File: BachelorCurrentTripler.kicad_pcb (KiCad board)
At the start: 2 copper layers, 132.3 x 99.3 mm, 54 parts, among them Q13 C2M0025120D, Q14 C2M0025120D, Q15 C2M0025120D, Q16 C2M0025120D, Q7 C2M0025120D, Q8 C2M0025120D, U1 STDriveG600, U2 STDriveG600, U3 STDriveG600

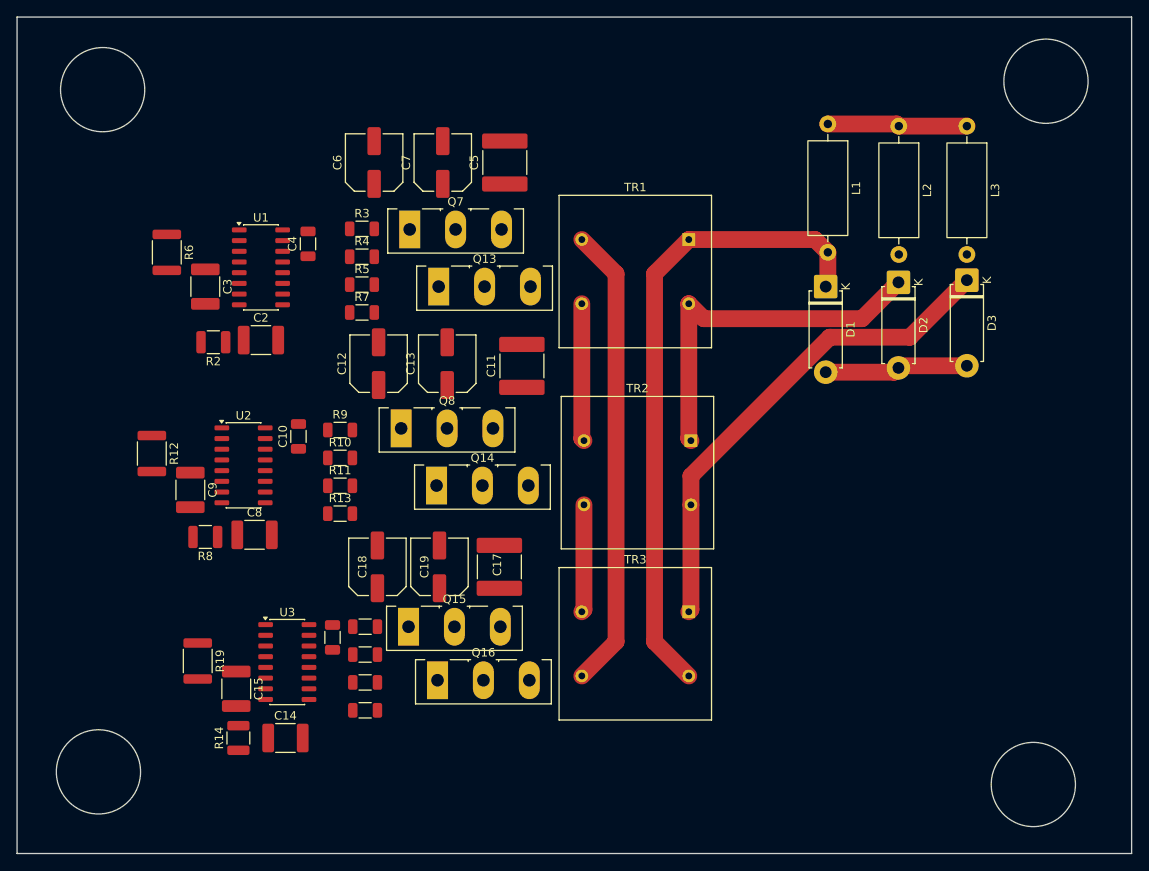
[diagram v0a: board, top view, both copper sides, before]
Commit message: intial pcb layout
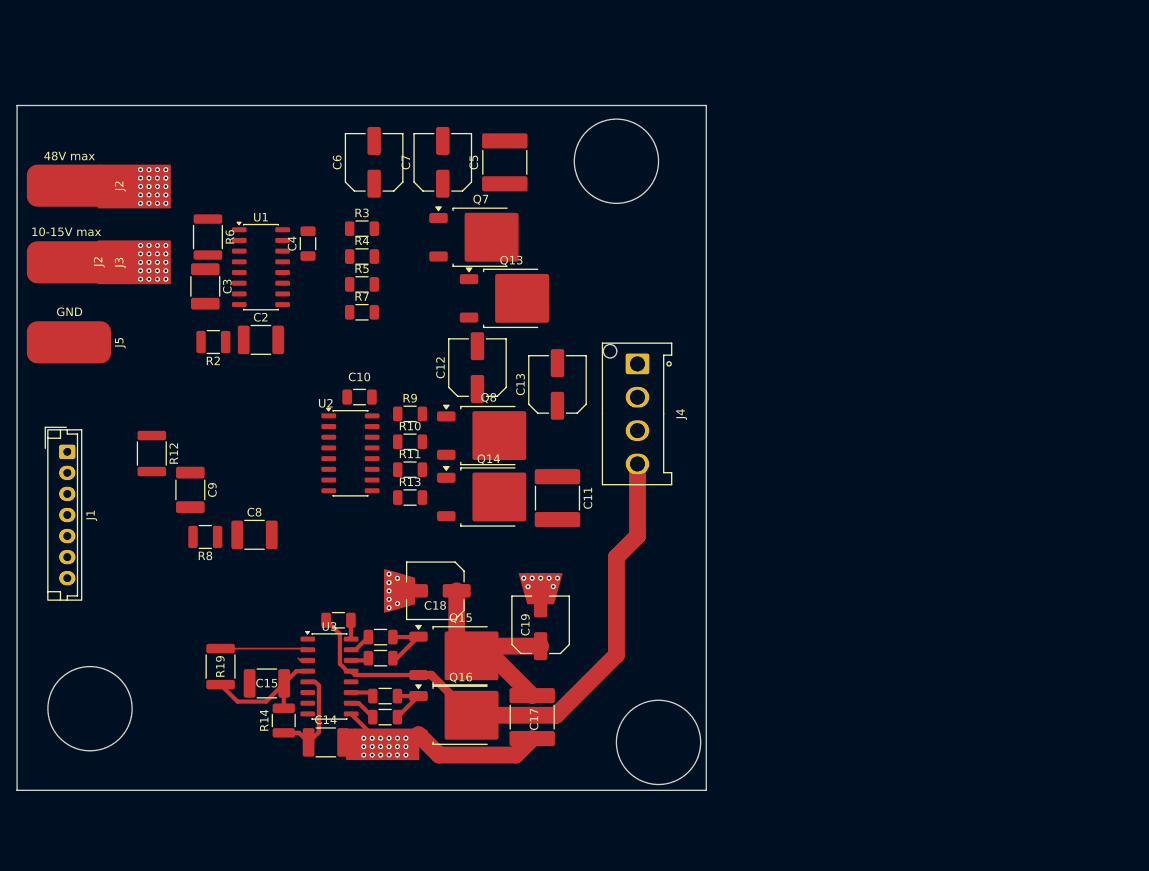
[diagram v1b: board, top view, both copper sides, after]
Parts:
- removed D1, D2, D3: D, Diode_THT:D_5W_P10.16mm_Horizontal
- removed L1, L2, L3: L, Inductor_THT:L_Axial_L11.0mm_D4.5mm_P15.24mm_Horizontal_Fastron_MECC
- removed TR1, TR2, TR3: 48:2, Transformer_THT:Transformer_NF_ETAL_1-1_P1200
- added J1: Conn_01x07_Pin, Connector_JST:JST_EH_B7B-EH-A_1x07_P2.50mm_Vertical, F.Cu at (90.8, 107.5)
- added J2: Conn_01x01_Pin, Connector_Wire:SolderWirePad_1x01_SMD_5x10mm, F.Cu at (91.0, 75.9)
- added J3: Conn_01x01_Pin, Connector_Wire:SolderWirePad_1x01_SMD_5x10mm, F.Cu at (91.0, 85.0)
- added J4: Conn_01x04_Socket, Connector_Hirose:Hirose_DF63M-4P-3.96DSA_1x04_P3.96mm_Vertical, F.Cu at (158.5, 97.1)
- added J5: Conn_01x01_Pin, Connector_Wire:SolderWirePad_1x01_SMD_5x10mm, F.Cu at (91.0, 94.5)
- Q13, Q14, Q15, Q16, Q7, Q8: footprint Package_TO_SOT_THT:TO-247-3_Vertical -> Package_TO_SOT_SMD:TO-252-2
- moved C17 18.3 mm to (146.0, 139.0), turned to -90 degrees
- moved C11 16.3 mm to (149.0, 113.0), turned to -90 degrees
- moved C19 13.8 mm to (147.0, 128.0)
- moved C13 13.3 mm to (149.0, 99.5)
- moved U2 12.8 mm to (124.4, 107.7)
- moved C12 11.7 mm to (139.5, 97.5)
- moved Q8 10.4 mm to (140.8, 105.6)
- moved Q13 8.76 mm to (143.5, 89.3)
- moved C10 8.63 mm to (125.5, 101.0), turned to 0 degrees
- moved R10 8.53 mm to (131.5, 106.3)
- moved R11 8.53 mm to (131.5, 109.6)
- moved R13 8.53 mm to (131.5, 112.9)
- moved R9 8.53 mm to (131.5, 103.0)
- moved Q7 8.51 mm to (139.9, 82.0)
- moved C18 7.44 mm to (134.5, 124.0), turned to 180 degrees
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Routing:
- net +48V: track 0.00 -> 128.9 mm, vias 0 -> 20
- net +12V: track 0.00 -> 80.6 mm, vias 0 -> 20
- net /Transformer/SecondaryA: track 76.5 -> 0.00 mm
- net /Transformer/SecondaryC: track 58.6 -> 0.00 mm
- net /PhaseC/COUT: track 12.8 -> 68.4 mm
- net /PhaseA/AOUT: track 55.2 -> 0.00 mm
- net /Transformer/SecondaryB: track 43.8 -> 0.00 mm
- net +1V2: track 16.6 -> 0.00 mm
- net /PhaseB/BOUT: track 16.4 -> 0.00 mm
- net /PhaseC/PVCC: track 0.00 -> 12.2 mm
- net Net-(U3-SD): track 0.00 -> 10.4 mm
- net Net-(Q15-G): track 0.00 -> 7.16 mm
- net Net-(Q16-G): track 0.00 -> 6.04 mm
- net GND: track 17.1 -> 22.4 mm, vias 0 -> 32
- net Net-(U3-LOFF): track 0.00 -> 3.26 mm
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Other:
- board size 132.3 x 99.3 mm -> 81.8 x 81.3 mm
- copper layers 2 -> 4
- board text added: "10-15V max"
- board text added: "48V max"
- board text added: "GND"
- board text added: "J2"
